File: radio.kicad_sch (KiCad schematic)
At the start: 7 parts, among them U5 ESP32-C6-WROOM-1

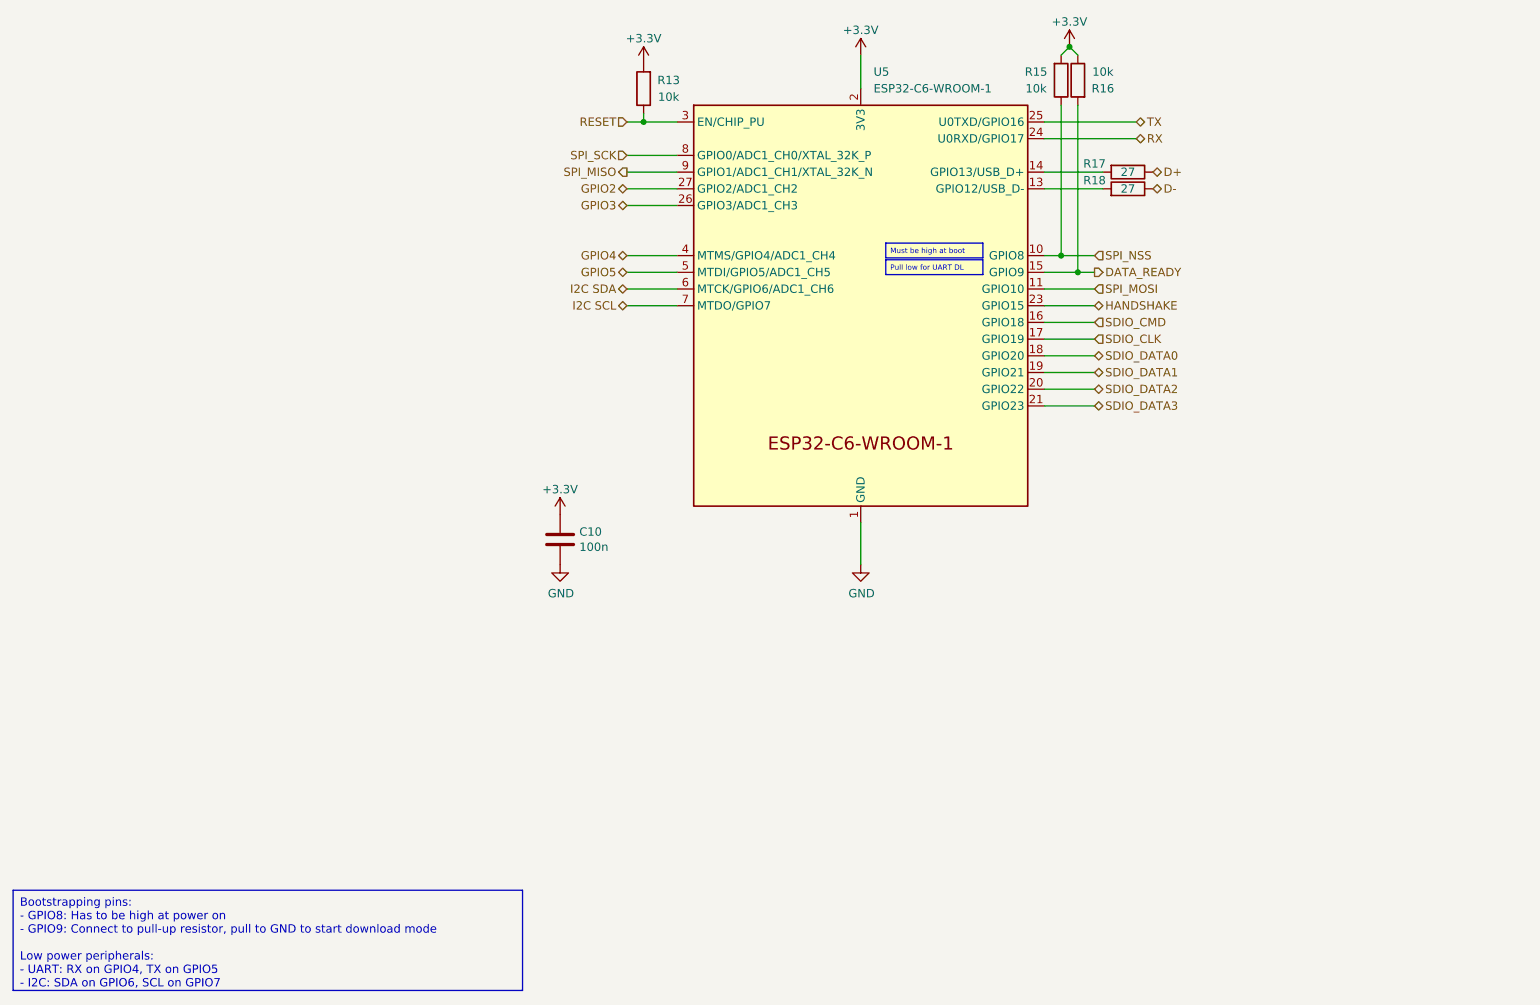
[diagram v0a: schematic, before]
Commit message: Work in progress
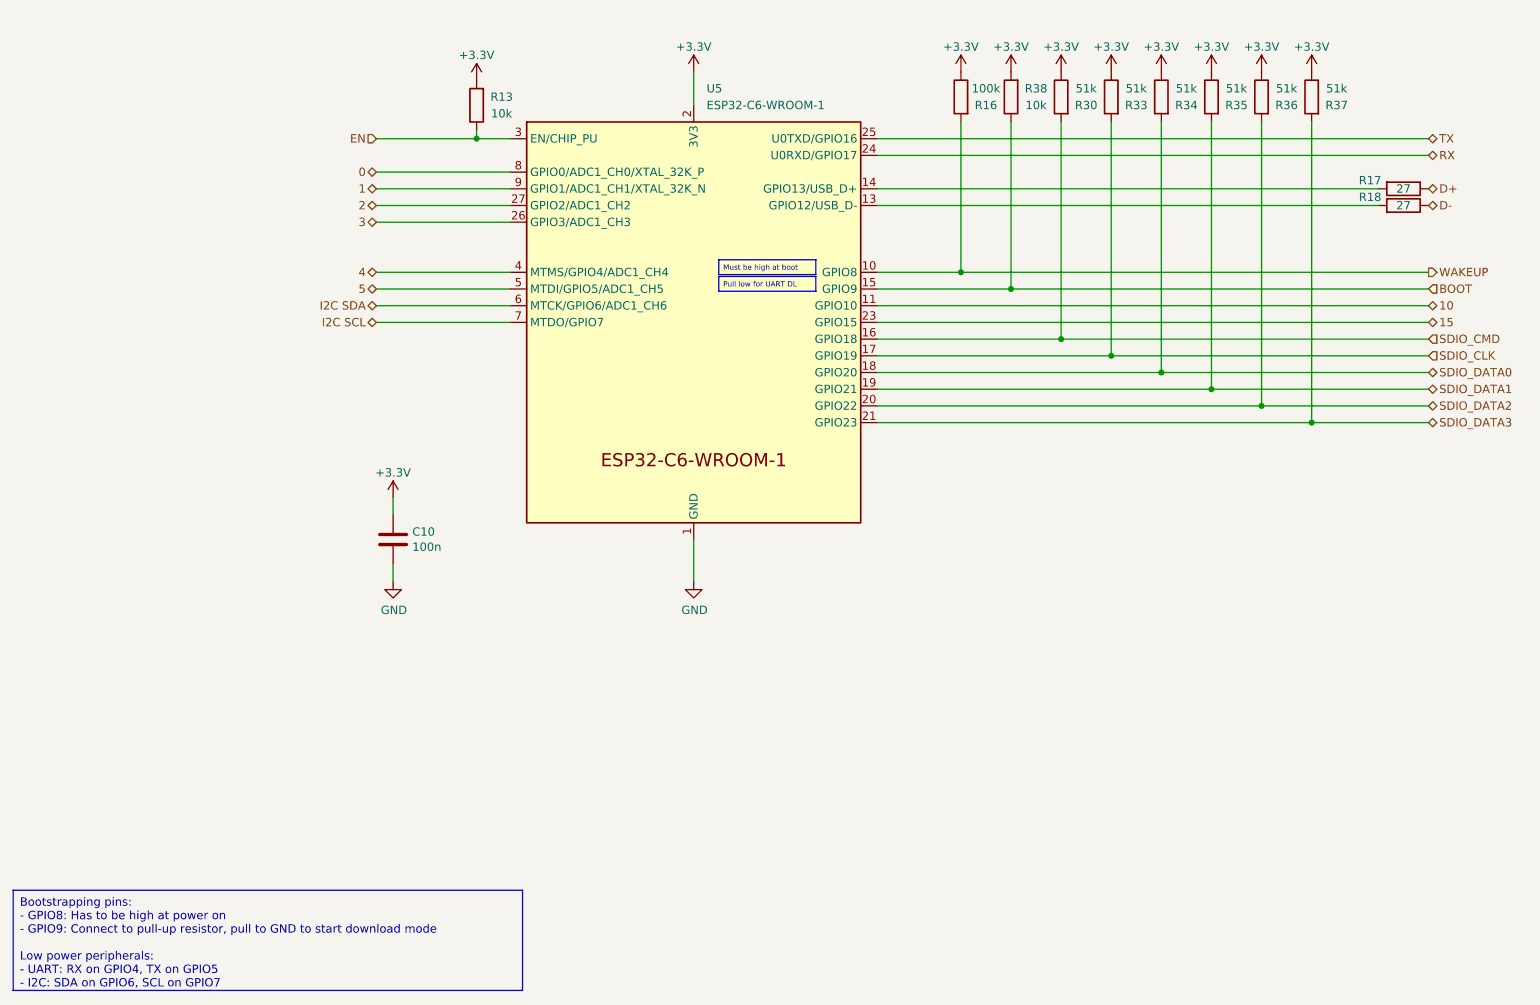
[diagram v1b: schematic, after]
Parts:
- removed R15: 10k, Resistor_SMD:R_0402_1005Metric, symbol symbols:R
- added R30, R33, R34, R35, R36, R37: 51k, Resistor_SMD:R_0402_1005Metric, symbol symbols:R
- added R38: 10k, Resistor_SMD:R_0402_1005Metric, symbol symbols:R
- R16: value 10k -> 100k; LCSC C25744 -> (none)
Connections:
- net +3.3V: now also R30.1, R33.1, R34.1, R35.1, R36.1, R37.1, R38.2
- net SDIO_CLK: now also R33.2
- net SDIO_CMD: now also R30.2
- net SDIO_DATA0: now also R34.2
- net SDIO_DATA1: now also R35.2
- net SDIO_DATA2: now also R36.2
- net SDIO_DATA3: now also R37.2
- net DATA_READY renamed BOOT
- net BOOT: now also R38.1; no longer R16.2
- net GPIO2 renamed 2
- net GPIO3 renamed 3
- net GPIO4 renamed 4
- net GPIO5 renamed 5
- net HANDSHAKE renamed 15
- net RESET renamed EN
- net SPI_MISO renamed 1
- net SPI_MOSI renamed 10
- net SPI_NSS renamed WAKEUP
- net WAKEUP: now also R16.2
- net SPI_SCK renamed 0
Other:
- moved on the sheet: C10, R13, R16, R17, R18, U5
